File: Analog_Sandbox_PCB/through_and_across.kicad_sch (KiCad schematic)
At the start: 10 parts, among them J1 PAD, J2 PAD, J3 PAD

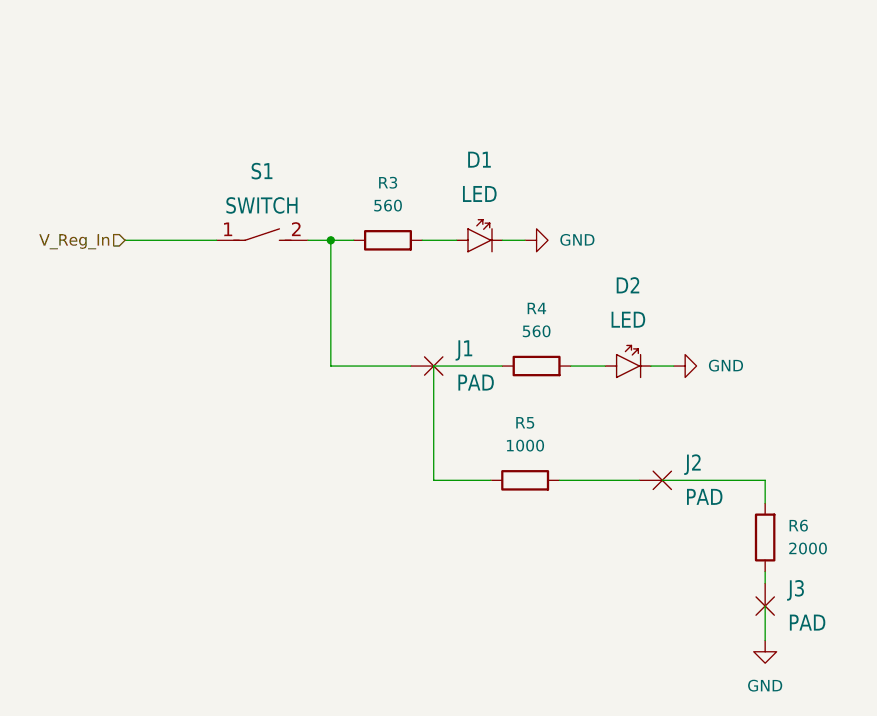
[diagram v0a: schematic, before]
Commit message: slight update
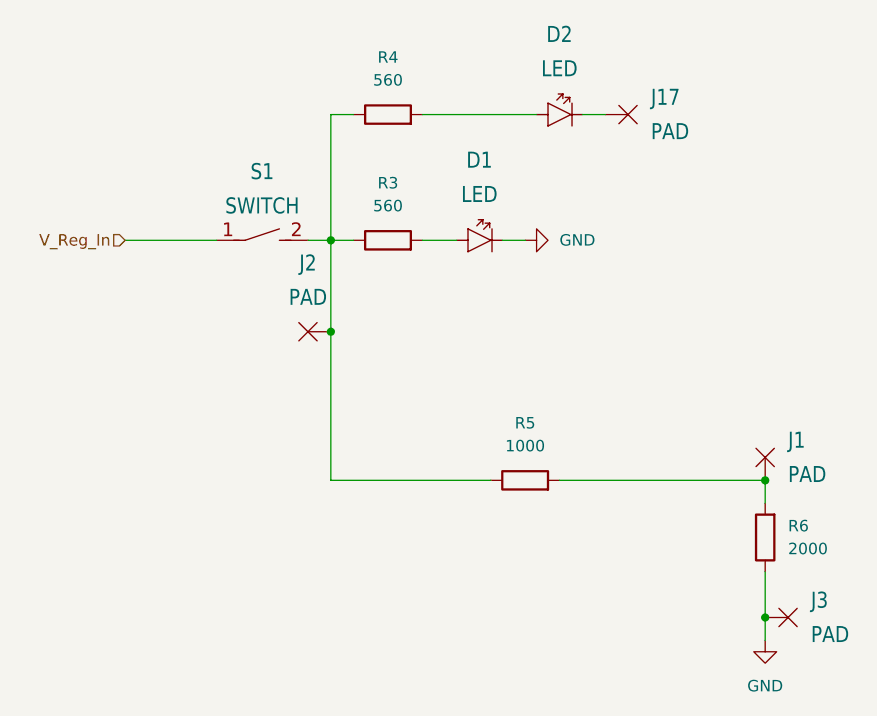
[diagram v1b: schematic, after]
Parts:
- added J17: PAD, TestPoint:TestPoint_Pad_2.5x2.5mm, symbol Analog_Sandbox_PCB-eagle-import:PAD
- J1: footprint TestPoint:TestPoint_Loop_D2.50mm_Drill1.0mm -> TestPoint:TestPoint_Pad_2.5x2.5mm
- J2, J3: footprint Analog_Sandbox_PCB:2.54_1.0 -> TestPoint:TestPoint_Pad_2.5x2.5mm
- R3, R4, R5, R6: footprint Resistor_SMD:R_2010_5025Metric_Pad1.40x2.65mm_HandSolder -> Resistor_SMD:R_1206_3216Metric
- S1: footprint Analog_Sandbox_PCB:DS-01 -> Button_Switch_THT:SW_DIP_SPSTx01_Slide_9.78x4.72mm_W7.62mm_P2.54mm
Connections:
- net GND: now also J3.1 (P), R6.1; no longer D2.C
- net at R4.1, R5.1: now also J2.1 (P), R3.1, S1.2
- net at R5.2: now also J1.1 (P), R6.2; no longer J2.1 (P)
- new net: D2.C, J17.1 (P)
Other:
- moved on the sheet: D2, R4

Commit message: All Circuits Added, Layout Almost done
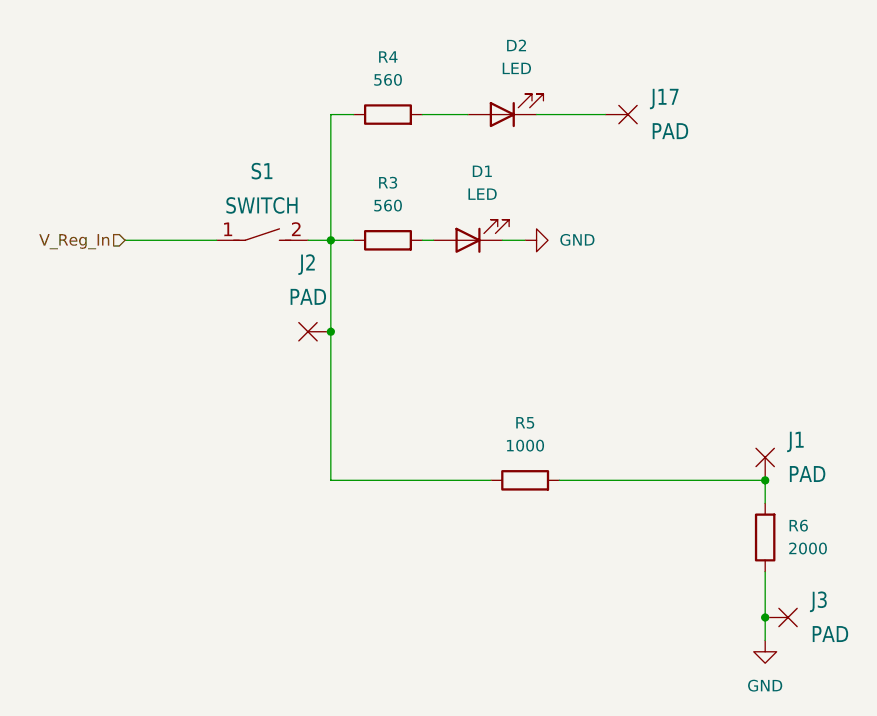
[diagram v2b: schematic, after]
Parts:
- removed D1, D2: LED, Diode_SMD:D_2010_5025Metric_Pad1.52x2.65mm_HandSolder, symbol Analog_Sandbox_PCB-eagle-import:CHIP-FLAT-Y_0603-0.35MM
- added D1, D2: LED, Diode_SMD:D_1206_3216Metric, symbol Device:LED
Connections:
- net GND: now also D1.1 (K)
- net at R4.2: now also D2.2 (A)
- net at J17.1 (P): now also D2.1 (K)
- net at R3.2: now also D1.2 (A)
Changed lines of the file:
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@@
 	(wire
 		(pts
-			(xy 116.84 21.59) (xy 119.38 21.59)
+			(xy 99.06 21.59) (xy 104.14 21.59)
+		)
+		(stroke
+			(width 0)
+			(type default)
+		)
+	)
+	(wire
+		(pts
+			(xy 107.95 35.56) (xy 110.49 35.56)
 		)
 		(stroke
@@
 	(wire
 		(pts
-			(xy 99.06 21.59) (xy 111.76 21.59)
-		)
-		(stroke
-			(width 0)
-			(type default)
-		)
-	)
-	(wire
-		(pts
 			(xy 114.3 62.23) (xy 137.16 62.23)
 		)
@@
 	(wire
 		(pts
+			(xy 111.76 21.59) (xy 119.38 21.59)
+		)
+		(stroke
+			(width 0)
+			(type default)
+		)
+	)
+	(wire
+		(pts
 			(xy 88.9 62.23) (xy 88.9 45.72)
 		)
@@
 	(wire
 		(pts
+			(xy 99.06 35.56) (xy 100.33 35.56)
+		)
+		(stroke
+			(width 0)
+			(type default)
+		)
+	)
+	(wire
+		(pts
 			(xy 88.9 21.59) (xy 88.9 35.56)
-		)
-		(stroke
-			(width 0)
-			(type default)
-		)
-	)
-	(wire
-		(pts
-			(xy 110.49 35.56) (xy 107.95 35.56)
-		)
-		(stroke
-			(width 0)
-			(type default)
-		)
-	)
-	(wire
-		(pts
-			(xy 99.06 35.56) (xy 102.87 35.56)
 		)
 		(stroke
@@
 	)
 	(symbol
-		(lib_id "Analog_Sandbox_PCB-eagle-import:CHIP-FLAT-Y_0603-0.35MM")
-		(at 114.3 21.59 0)
-		(unit 1)
-		(exclude_from_sim no)
-		(in_bom yes)
-		(on_board yes)
-		(dnp no)
-		(fields_autoplaced yes)
-		(property "Reference" "D2"
-			(at 114.3 12.7 0)
-			(effects
-				(font
-					(size 1.778 1.5113)
+		(lib_id "Device:LED")
+		(at 104.14 35.56 180)
+		(unit 1)
+		(exclude_from_sim no)
+		(in_bom yes)
+		(on_board yes)
+		(dnp no)
+		(fields_autoplaced yes)
+		(property "Reference" "D1"
+			(at 105.7275 27.94 0)
+			(effects
+				(font
+					(size 1.27 1.27)
 				)
 			)
 		)
 		(property "Value" "LED"
-			(at 114.3 16.51 0)
-			(effects
-				(font
-					(size 1.778 1.5113)
-				)
-			)
-		)
-		(property "Footprint" "Diode_SMD:D_2010_5025Metric_Pad1.52x2.65mm_HandSolder"
-			(at 114.3 21.59 0)
-			(effects
-				(font
-					(size 1.27 1.27)
-				)
-				(hide yes)
-			)
-		)
-		(property "Datasheet" ""
-			(at 114.3 21.59 0)
-			(effects
-				(font
-					(size 1.27 1.27)
-				)
-				(hide yes)
-			)
-		)
-		(property "Description" "Yellow LED - Generic"
-			(at 114.3 21.59 0)
-			(effects
-				(font
-					(size 1.27 1.27)
-				)
-				(hide yes)
-			)
-		)
-		(pin "A"
-		)
-		(pin "C"
-		)
-		(instances
-			(project "Analog_Sandbox_PCB"
-				(path "/ac750111-a1db-4b3c-a106-e1424e47aebb/5f1ad39e-0f17-4880-9544-2cfbd63a3a10"
-					(reference "D2")
-					(unit 1)
-				)
-			)
-		)
-	)
-	(symbol
-		(lib_id "Analog_Sandbox_PCB-eagle-import:CHIP-FLAT-Y_0603-0.35MM")
-		(at 105.41 35.56 0)
-		(unit 1)
-		(exclude_from_sim no)
-		(in_bom yes)
-		(on_board yes)
-		(dnp no)
-		(fields_autoplaced yes)
-		(property "Reference" "D1"
-			(at 105.41 26.67 0)
-			(effects
-				(font
-					(size 1.778 1.5113)
-				)
-			)
-		)
-		(property "Value" "LED"
-			(at 105.41 30.48 0)
-			(effects
-				(font
-					(size 1.778 1.5113)
-				)
-			)
-		)
-		(property "Footprint" "Diode_SMD:D_2010_5025Metric_Pad1.52x2.65mm_HandSolder"
-			(at 105.41 35.56 0)
-			(effects
-				(font
-					(size 1.27 1.27)
-				)
-				(hide yes)
-			)
-		)
-		(property "Datasheet" ""
-			(at 105.41 35.56 0)
-			(effects
-				(font
-					(size 1.27 1.27)
-				)
-				(hide yes)
-			)
-		)
-		(property "Description" "Yellow LED - Generic"
-			(at 105.41 35.56 0)
-			(effects
-				(font
-					(size 1.27 1.27)
-				)
-				(hide yes)
-			)
-		)
-		(pin "A"
-		)
-		(pin "C"
+			(at 105.7275 30.48 0)
+			(effects
+				(font
+					(size 1.27 1.27)
+				)
+			)
+		)
+		(property "Footprint" "Diode_SMD:D_1206_3216Metric"
+			(at 104.14 35.56 0)
+			(effects
+				(font
+					(size 1.27 1.27)
+				)
+				(hide yes)
+			)
+		)
+		(property "Datasheet" "~"
+			(at 104.14 35.56 0)
+			(effects
+				(font
+					(size 1.27 1.27)
+				)
+				(hide yes)
+			)
+		)
+		(property "Description" "Light emitting diode"
+			(at 104.14 35.56 0)
+			(effects
+				(font
+					(size 1.27 1.27)
+				)
+				(hide yes)
+			)
+		)
+		(property "Sim.Pins" "1=K 2=A"
+			(at 104.14 35.56 0)
+			(effects
+				(font
+					(size 1.27 1.27)
+				)
+				(hide yes)
+			)
+		)
+		(pin "1"
+		)
+		(pin "2"
 		)
 		(instances
@@
 					(unit 1)
 				)
+			)
+		)
+	)
+	(symbol
+		(lib_id "Device:LED")
+		(at 107.95 21.59 180)
+		(unit 1)
+		(exclude_from_sim no)
+		(in_bom yes)
+		(on_board yes)
+		(dnp no)
+		(fields_autoplaced yes)
+		(property "Reference" "D2"
+			(at 109.5375 13.97 0)
+			(effects
+				(font
+					(size 1.27 1.27)
+				)
+			)
+		)
+		(property "Value" "LED"
+			(at 109.5375 16.51 0)
+			(effects
+				(font
+					(size 1.27 1.27)
+				)
+			)
+		)
+		(property "Footprint" "Diode_SMD:D_1206_3216Metric"
+			(at 107.95 21.59 0)
+			(effects
+				(font
+					(size 1.27 1.27)
+				)
+				(hide yes)
+			)
+		)
+		(property "Datasheet" "~"
+			(at 107.95 21.59 0)
+			(effects
+				(font
+					(size 1.27 1.27)
+				)
+				(hide yes)
+			)
+		)
+		(property "Description" "Light emitting diode"
+			(at 107.95 21.59 0)
+			(effects
+				(font
+					(size 1.27 1.27)
+				)
+				(hide yes)
+			)
+		)
+		(property "Sim.Pins" "1=K 2=A"
+			(at 107.95 21.59 0)
+			(effects
+				(font
+					(size 1.27 1.27)
+				)
+				(hide yes)
+			)
+		)
+		(pin "1"
+		)
+		(pin "2"
+		)
+		(instances
+			(project "Analog_Sandbox_PCB"
+				(path "/ac750111-a1db-4b3c-a106-e1424e47aebb/5f1ad39e-0f17-4880-9544-2cfbd63a3a10"
+					(reference "D2")
+					(unit 1)
+				)
